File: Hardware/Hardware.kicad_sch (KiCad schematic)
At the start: 30 parts, among them J1 USB_C_Receptacle_USB2.0_16P, J2 Conn_01x06, J3 Conn_01x04, Q1 BSS138, Q2 BSS138, U2 CH340C, U4 ESP32-WROOM-32, U5 AMS1117-3.3

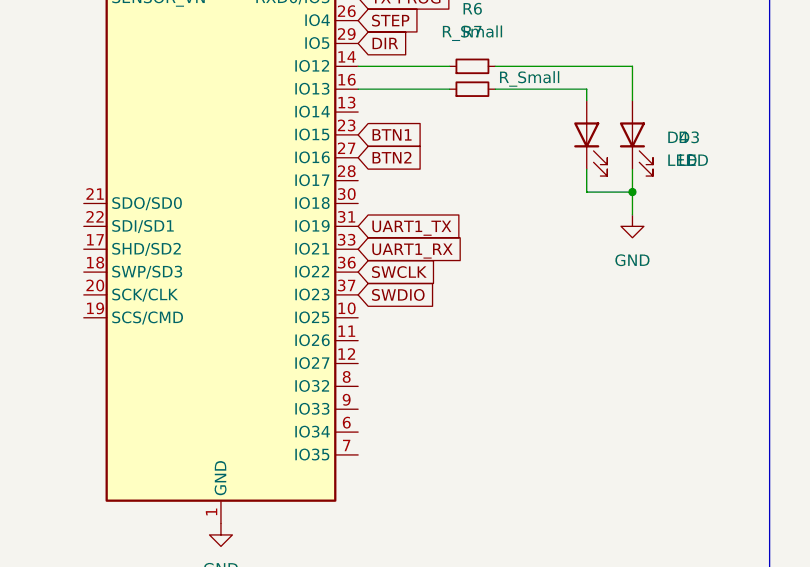
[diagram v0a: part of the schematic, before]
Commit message: finish pcb wiring
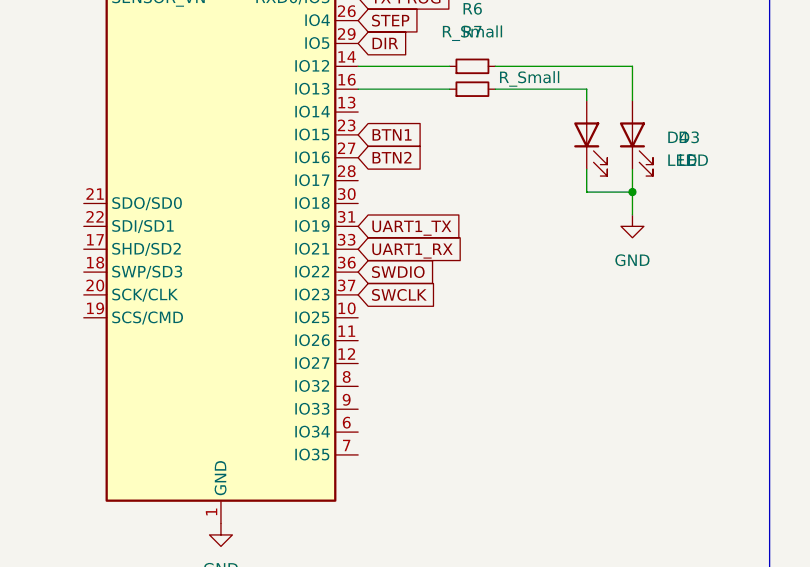
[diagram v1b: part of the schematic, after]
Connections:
- net SWCLK: now also U4.37 (IO23); no longer U4.36 (IO22)
- net SWDIO: now also U4.36 (IO22); no longer U4.37 (IO23)
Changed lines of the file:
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@@
+		)
+	)
+	(global_label "SWCLK"
+		(shape input)
+		(at 110.49 111.76 0)
+		(fields_autoplaced yes)
+		(effects
+			(font
+				(size 1.27 1.27)
+			)
+			(justify left)
+		)
+		(property "Intersheetrefs" "${INTERSHEET_REFS}"
+			(at 119.7042 111.76 0)
+			(hide yes)
+			(show_name no)
+			(do_not_autoplace no)
+			(effects
+				(font
+					(size 1.27 1.27)
+				)
+				(justify left)
+			)
 		)
 	)
@@
 		(property "Intersheetrefs" "${INTERSHEET_REFS}"
 			(at 122.4861 104.14 0)
-			(hide yes)
-			(show_name no)
-			(do_not_autoplace no)
-			(effects
-				(font
-					(size 1.27 1.27)
-				)
-				(justify left)
-			)
-		)
-	)
-	(global_label "SWDIO"
-		(shape input)
-		(at 110.49 111.76 0)
-		(fields_autoplaced yes)
-		(effects
-			(font
-				(size 1.27 1.27)
-			)
-			(justify left)
-		)
-		(property "Intersheetrefs" "${INTERSHEET_REFS}"
-			(at 119.3414 111.76 0)
 			(hide yes)
 			(show_name no)
@@
 		)
 	)
+	(global_label "SWDIO"
+		(shape input)
+		(at 110.49 109.22 0)
+		(fields_autoplaced yes)
+		(effects
+			(font
+				(size 1.27 1.27)
+			)
+			(justify left)
+		)
+		(property "Intersheetrefs" "${INTERSHEET_REFS}"
+			(at 119.3414 109.22 0)
+			(hide yes)
+			(show_name no)
+			(do_not_autoplace no)
+			(effects
+				(font
+					(size 1.27 1.27)
+				)
+				(justify left)
+			)
+		)
+	)
 	(global_label "TX-PROG"
 		(shape input)
@@
 			(hide yes)
 			(show_name no)
-			(do_not_autoplace no)
-			(effects
-				(font
-					(size 1.27 1.27)
-				)
-				(justify left)
-			)
-		)
-	)
-	(global_label "SWCLK"
-		(shape input)
-		(at 110.49 109.22 0)
-		(fields_autoplaced yes)
-		(effects
-			(font
-				(size 1.27 1.27)
-			)
-			(justify left)
-		)
-		(property "Intersheetrefs" "${INTERSHEET_REFS}"
-			(at 119.7042 109.22 0)
-			(hide yes)
-			(show_name no)
